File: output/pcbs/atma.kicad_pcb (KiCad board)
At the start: 2 copper layers, 99.8 x 100 mm, 24 parts

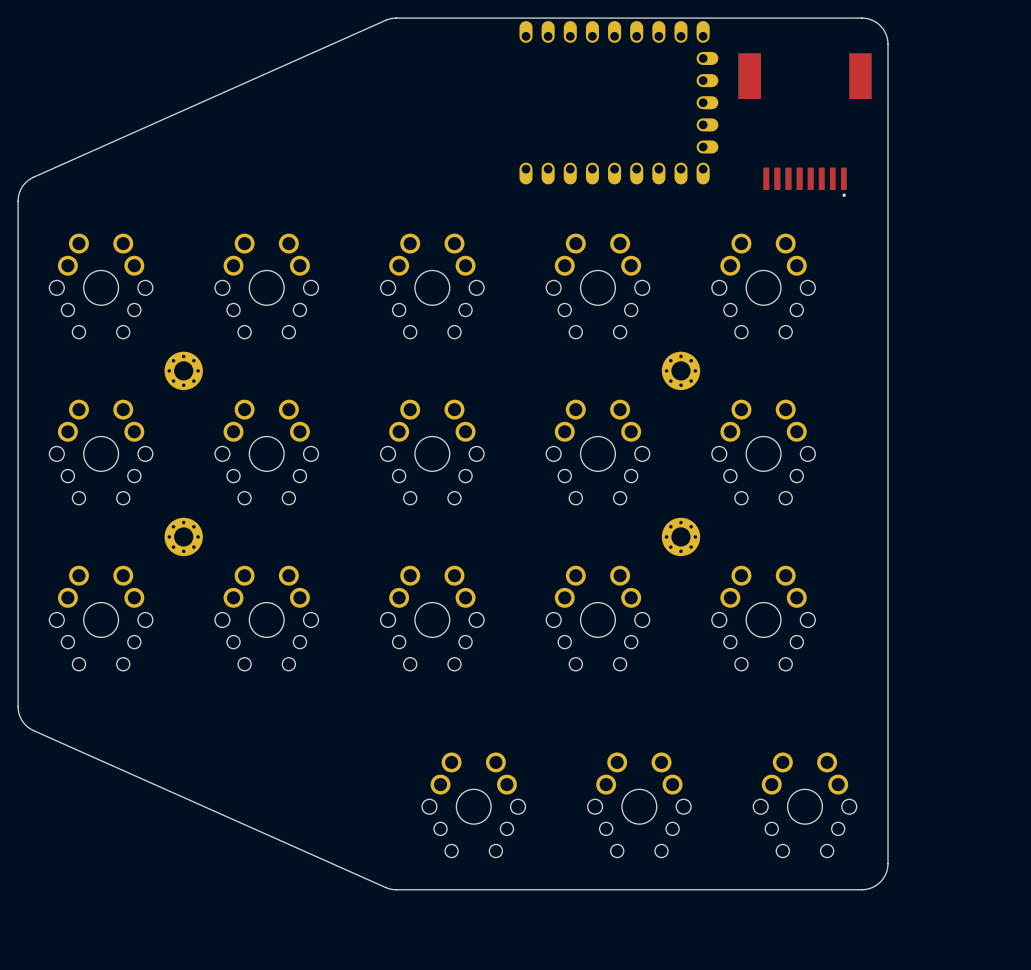
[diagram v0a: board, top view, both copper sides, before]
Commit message: more ergonomic 36-key version
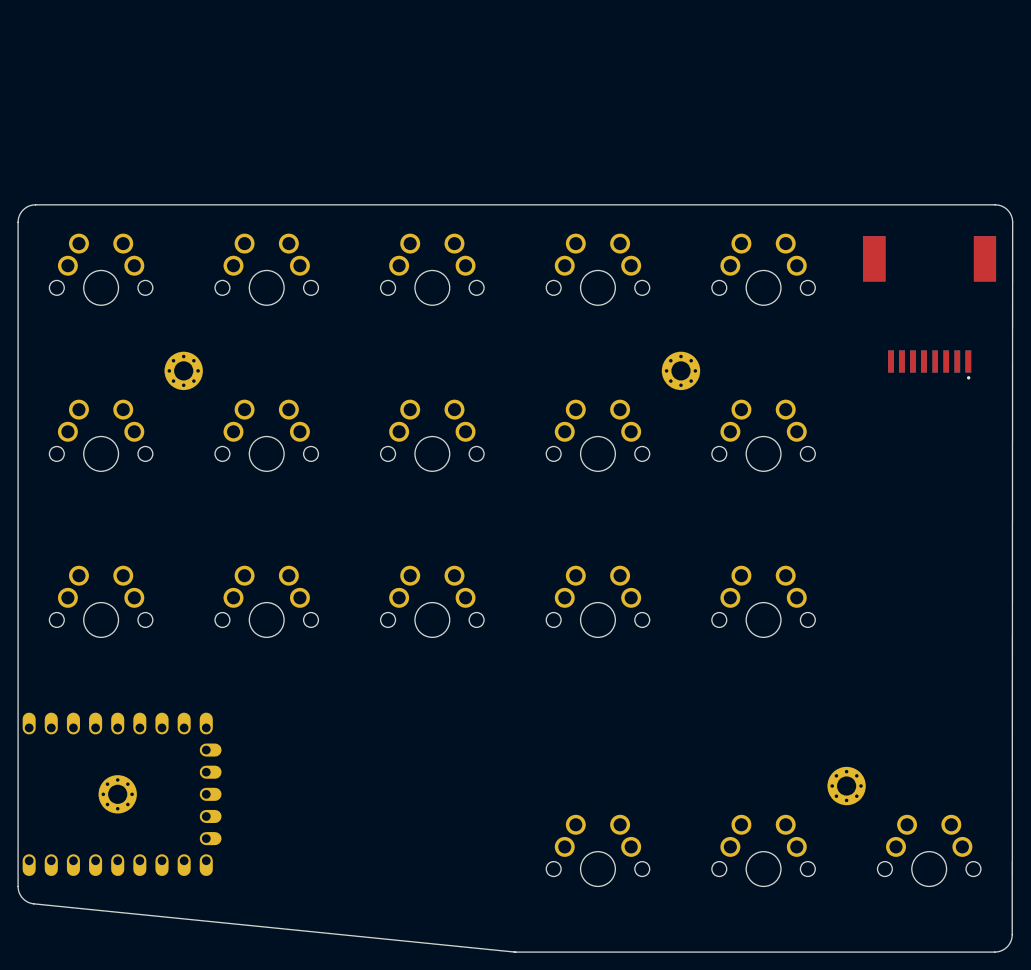
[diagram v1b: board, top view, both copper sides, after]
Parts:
- moved ? 97.7 mm to (154.3, 172.4)
- moved _6 71.0 mm to (154.3, 172.4)
- moved _4 60.1 mm to (218.9, 123.8)
- moved _5 51.3 mm to (237.9, 171.4)
- moved ? 25.4 mm to (247.5, 121.9)
- moved S16 15.9 mm to (209.4, 181.0)
- moved S17 15.9 mm to (228.4, 181.0)
- moved S18 15.9 mm to (247.4, 181.0)
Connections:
- ? pad 1: matrix_pinky_bottom -> matrix_pinky_top
- ? pad 10: GP9 -> matrix_index_top
- ? pad 11: matrix_middle_top -> matrix_index_home
- ? pad 12: matrix_inner_bottom -> matrix_index_bottom
- ? pad 13: matrix_inner_home -> GP12
- ? pad 14: matrix_inner_top -> GP13
- ? pad 15: matrix_index_top -> matrix_inner_bottom
- ? pad 16: matrix_index_home -> matrix_inner_home
- ? pad 17: matrix_index_bottom -> matrix_inner_top
- ? pad 18: thumbfan_far_home -> thumbfan_near_home
- ? pad 20: thumbfan_near_home -> thumbfan_far_home
- ? pad 3: matrix_pinky_top -> matrix_pinky_bottom
- ? pad 4: matrix_ring_top -> matrix_ring_bottom
- ? pad 6: matrix_ring_bottom -> matrix_ring_top
- ? pad 7: matrix_middle_bottom -> matrix_middle_top
- ? pad 9: GP8 -> matrix_middle_bottom
- ? pad 3: GP8 -> GP12
- ? pad 4: GP8 -> GP12
- ? pad 5: GP9 -> GP13
- ? pad 6: GP9 -> GP13
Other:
- board size 99.8 x 100 mm -> 114.1 x 85.7 mm

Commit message: outline tweaks
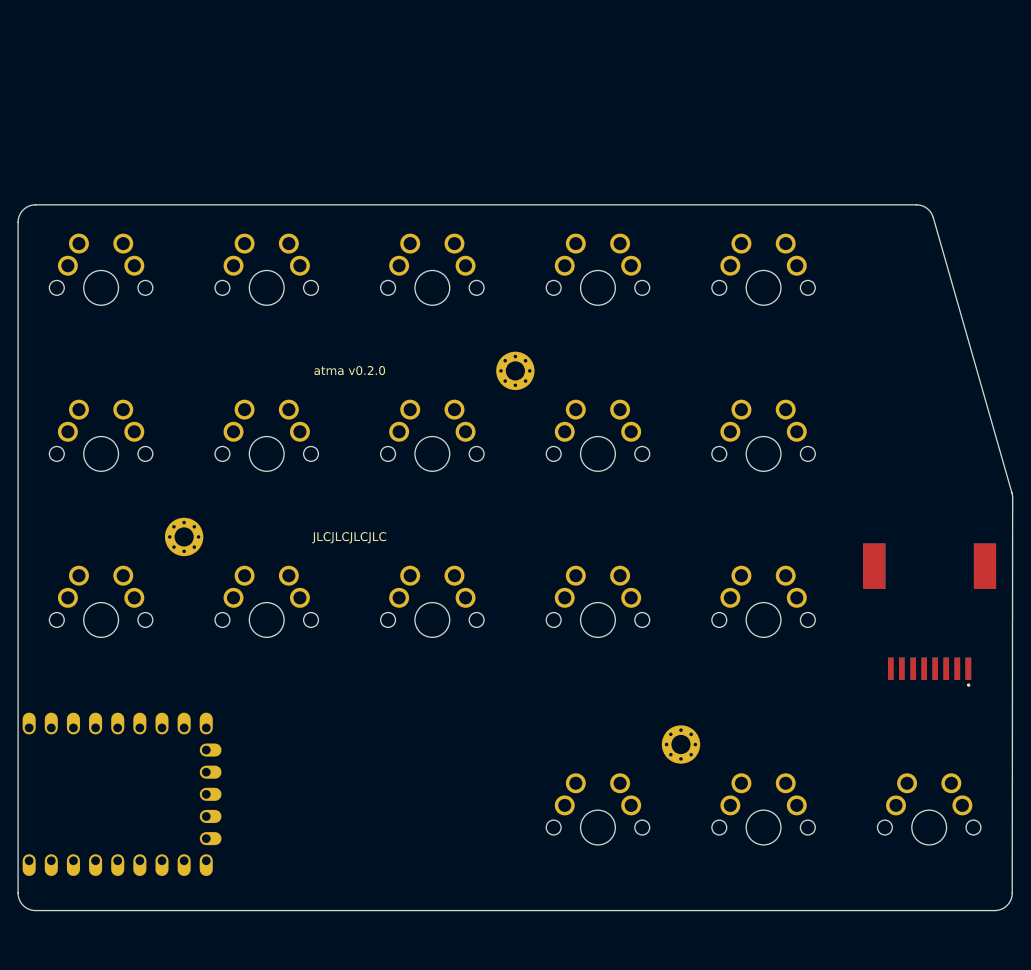
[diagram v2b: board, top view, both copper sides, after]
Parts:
- removed _6: , MountingHole_2.2mm_M2_Pad_Via
- moved ? 35.2 mm to (247.5, 157.2)
- moved _5 19.6 mm to (218.9, 166.7)
- moved _3 19.1 mm to (161.9, 142.9)
- moved _4 19.0 mm to (199.9, 123.8)
- moved S16 4.76 mm to (209.4, 176.2)
- moved S17 4.76 mm to (228.4, 176.2)
- moved S18 4.76 mm to (247.4, 176.2)
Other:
- board size 114.1 x 85.7 mm -> 114.1 x 81 mm
- board text added: "JLCJLCJLCJLC"
- board text added: "atma v0.2.0"
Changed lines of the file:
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@@
           )
       (module MX (layer F.Cu)
-      (at 209.4 180.975 0)
+      (at 209.4 176.2125 0)
       (fp_text reference "S16" (at 0 0) (layer F.SilkS) hide (effects (font (size 1.27 1.27) (thickness 0.15))))
       (fp_text value "" (at 0 0) (layer F.SilkS) hide (effects (font (size 1.27 1.27) (thickness 0.15))))
@@
           )
       (module MX (layer F.Cu)
-      (at 228.4 180.975 0)
+      (at 228.4 176.2125 0)
       (fp_text reference "S17" (at 0 0) (layer F.SilkS) hide (effects (font (size 1.27 1.27) (thickness 0.15))))
       (fp_text value "" (at 0 0) (layer F.SilkS) hide (effects (font (size 1.27 1.27) (thickness 0.15))))
@@
           )
       (module MX (layer F.Cu)
-      (at 247.4 180.975 0)
+      (at 247.4 176.2125 0)
       (fp_text reference "S18" (at 0 0) (layer F.SilkS) hide (effects (font (size 1.27 1.27) (thickness 0.15))))
       (fp_text value "" (at 0 0) (layer F.SilkS) hide (effects (font (size 1.27 1.27) (thickness 0.15))))
@@
     )
     (module "44144-0003" (layer F.Cu)
-      (at 247.45000000000002 121.91999999999999 180)
+      (at 247.45000000000002 157.1625 180)
       (fp_line (start -7.62 0) (end 7.62 0) (layer F.Fab) (width 0.2))
       (fp_line (start 7.62 0) (end 7.62 16.89) (layer F.Fab) (width 0.2))
@@
     )
     (module "MountingHole_2.2mm_M2_Pad_Via" (version 20210722) (generator pcbnew) (layer "F.Cu")
-      (at 161.875 123.82499999999999 0)
+      (at 161.925 142.875 0)
       (fp_text reference "_3" (at 0 -3.2) (layer "F.SilkS") hide
         (effects (font (size 1 1) (thickness 0.15)))
@@
     )
     (module "MountingHole_2.2mm_M2_Pad_Via" (version 20210722) (generator pcbnew) (layer "F.Cu")
-      (at 218.925 123.82499999999999 0)
+      (at 199.925 123.82499999999999 0)
       (fp_text reference "_4" (at 0 -3.2) (layer "F.SilkS") hide
         (effects (font (size 1 1) (thickness 0.15)))
@@
     )
     (module "MountingHole_2.2mm_M2_Pad_Via" (version 20210722) (generator pcbnew) (layer "F.Cu")
-      (at 237.925 171.45 0)
+      (at 218.925 166.6875 0)
       (fp_text reference "_5" (at 0 -3.2) (layer "F.SilkS") hide
         (effects (font (size 1 1) (thickness 0.15)))
@@
       (pad "1" thru_hole circle locked (at 0 -1.65) (size 0.7 0.7) (drill 0.4) (layers *.Cu *.Mask))
     )
-    (module "MountingHole_2.2mm_M2_Pad_Via" (version 20210722) (generator pcbnew) (layer "F.Cu")
-      (at 154.305 172.4025 0)
-      (fp_text reference "_6" (at 0 -3.2) (layer "F.SilkS") hide
-        (effects (font (size 1 1) (thickness 0.15)))
-      )
-      (fp_circle (center 0 0) (end 2.45 0) (layer "F.CrtYd") (width 0.05) (fill none))
-      (pad "1" thru_hole circle locked (at 1.166726 1.166726) (size 0.7 0.7) (drill 0.4) (layers *.Cu *.Mask))
-      (pad "1" thru_hole circle locked (at 0 0) (size 4.4 4.4) (drill 2.2) (layers *.Cu *.Mask))
-      (pad "1" thru_hole circle locked (at 0 1.65) (size 0.7 0.7) (drill 0.4) (layers *.Cu *.Mask))
-      (pad "1" thru_hole circle locked (at 1.166726 -1.166726) (size 0.7 0.7) (drill 0.4) (layers *.Cu *.Mask))
-      (pad "1" thru_hole circle locked (at -1.65 0) (size 0.7 0.7) (drill 0.4) (layers *.Cu *.Mask))
-      (pad "1" thru_hole circle locked (at -1.166726 -1.166726) (size 0.7 0.7) (drill 0.4) (layers *.Cu *.Mask))
-      (pad "1" thru_hole circle locked (at -1.166726 1.166726) (size 0.7 0.7) (drill 0.4) (layers *.Cu *.Mask))
-      (pad "1" thru_hole circle locked (at 1.65 0) (size 0.7 0.7) (drill 0.4) (layers *.Cu *.Mask))
-      (pad "1" thru_hole circle locked (at 0 -1.65) (size 0.7 0.7) (drill 0.4) (layers *.Cu *.Mask))
-    )
-            (gr_line (start 142.875 182.97549871897368) (end 142.875 106.77499999999999) (angle 90) (layer Edge.Cuts) (width 0.15))
-(gr_line (start 144.875 104.77499999999999) (end 254.97383309877515 104.77499999999999) (angle 90) (layer Edge.Cuts) (width 0.15))
-(gr_line (start 256.97383279871684 106.77616660005879) (end 256.92616584041997 188.5011665999773) (angle 90) (layer Edge.Cuts) (width 0.15))
-(gr_line (start 254.9261661404783 190.5) (end 199.9750127766405 190.5) (angle 90) (layer Edge.Cuts) (width 0.15))
-(gr_line (start 199.77548676770925 190.49002248907823) (end 144.67547399106874 184.96552120805188) (angle 90) (layer Edge.Cuts) (width 0.15))
+            (gr_text "atma v0.2.0" (at 180.925 123.82499999999999 0) (layer F.SilkS)
+                (effects (font (size 1 1) (thickness 0.15)) )
+            )
+            (gr_text "JLCJLCJLCJLC" (at 180.925 142.875 0) (layer F.SilkS)
+                (effects (font (size 1 1) (thickness 0.15)) )
+            )
+            (gr_line (start 142.875 183.7375) (end 142.875 106.77499999999999) (angle 90) (layer Edge.Cuts) (width 0.15))
+(gr_line (start 144.875 104.77499999999999) (end 245.9413971571429 104.77499999999999) (angle 90) (layer Edge.Cuts) (width 0.15))
+(gr_line (start 247.8644450760108 106.22555776603781) (end 256.8977538164621 137.84213835761727) (angle 90) (layer Edge.Cuts) (width 0.15))
+(gr_line (start 256.97470479748904 138.39368039168767) (end 256.92709753301824 183.73959980011568) (angle 90) (layer Edge.Cuts) (width 0.15))
+(gr_line (start 144.875 185.7375) (end 254.92709863312336 185.7375) (angle 90) (layer Edge.Cuts) (width 0.15))
 (gr_arc (start 144.875 106.77499999999999) (end 144.875 104.77499999999999) (angle -90) (layer Edge.Cuts) (width 0.15))
-(gr_arc (start 254.97383309877515 106.77499999999999) (end 256.97383279877516 106.7761666) (angle -90.03342063109807) (layer Edge.Cuts) (width 0.15))
-(gr_arc (start 254.9261661404783 188.5) (end 254.9261661404783 190.5) (angle -89.96657937123672) (layer Edge.Cuts) (width 0.15))
-(gr_arc (start 199.9750127766405 188.5) (end 199.77548677664052 190.4900225) (angle -5.725523291754314) (layer Edge.Cuts) (width 0.15))
-(gr_arc (start 144.875 182.97549871897368) (end 142.875 182.97549871897368) (angle -84.27447670824557) (layer Edge.Cuts) (width 0.15))
+(gr_arc (start 245.9413971571429 106.77499999999999) (end 247.8644450571429 106.22555779999999) (angle -74.05460488609745) (layer Edge.Cuts) (width 0.15))
+(gr_arc (start 254.97470589759416 138.39158059157955) (end 256.97470479759414 138.39368039157955) (angle -16.00554996689867) (layer Edge.Cuts) (width 0.15))
+(gr_arc (start 254.92709863312336 183.73749999998836) (end 254.92709863312336 185.73749999998836) (angle -89.93984514645598) (layer Edge.Cuts) (width 0.15))
+(gr_arc (start 144.875 183.7375) (end 142.875 183.7375) (angle -90) (layer Edge.Cuts) (width 0.15))
 )
